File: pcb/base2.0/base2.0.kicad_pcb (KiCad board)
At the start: 4 copper layers, 24 x 24 mm, 33 parts, among them J1 Conn_01x01_Male, J2 Conn_01x01_Male, J3 Conn_ARM_JTAG_SWD_10, J4 Conn_01x02_Male, Q1 BSS123, U1 STM32G431CBU6, U2 tile, U3 AP2210-33, U4 LSM6DS3, U5 AP2210-5

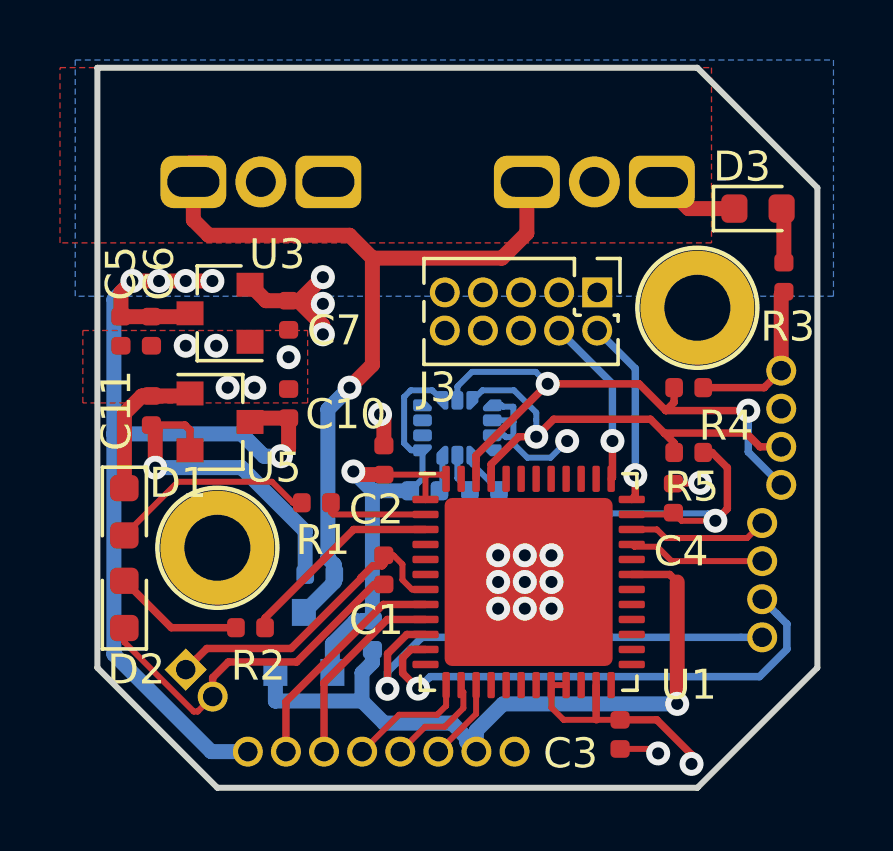
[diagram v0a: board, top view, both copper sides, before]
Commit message: added another pcbs
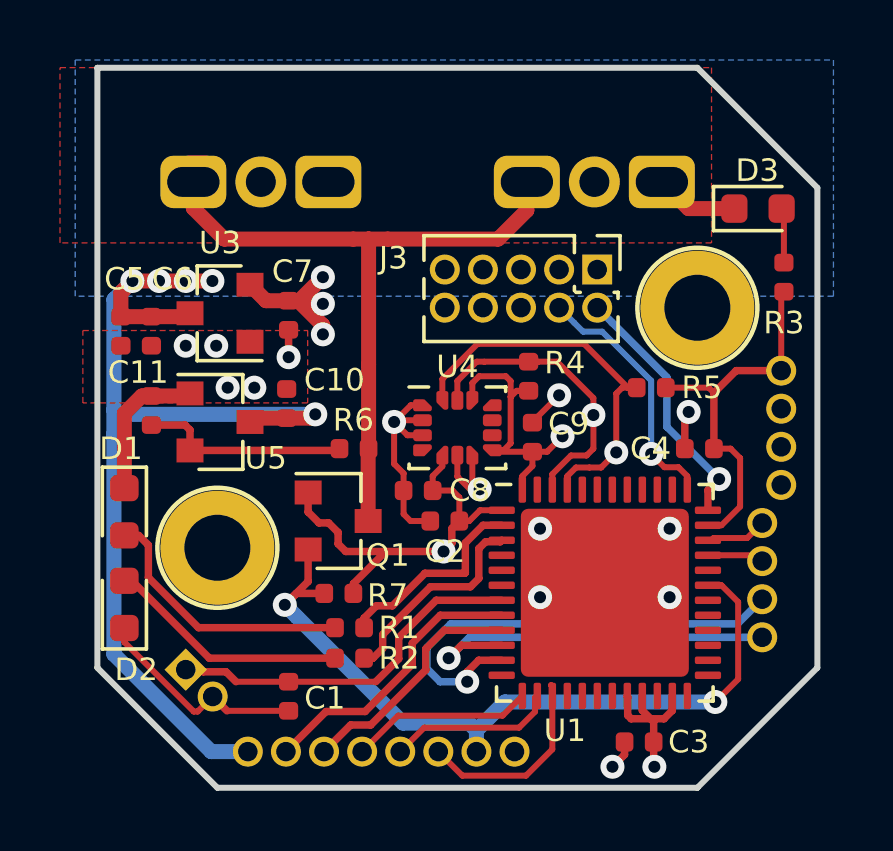
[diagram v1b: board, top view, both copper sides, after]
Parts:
- C8, C9, Q1, R6, R7, U4: moved to F.Cu
- moved R4 5.35 mm to (206.4, 97.3), turned to 90 degrees
- moved C1 5.28 mm to (198.4, 108.0)
- moved R6 4.34 mm to (200.6, 99.7)
- moved R1 4.31 mm to (200.4, 105.7)
- moved Q1 4.21 mm to (200.0, 102.1), turned to 0 degrees
- moved C9 4.00 mm to (206.5, 99.3), turned to 270 degrees
- moved R2 3.45 mm to (200.4, 106.7)
- moved C2 2.87 mm to (203.6, 102.1), turned to 180 degrees
- moved U1 2.57 mm to (208.9, 104.5)
- moved R5 2.49 mm to (210.5, 97.7)
- moved C8 2.21 mm to (202.7, 101.1)
- moved C4 1.86 mm to (212.1, 99.7), turned to 180 degrees
- moved R7 1.79 mm to (200.0, 104.5), turned to 180 degrees
- moved J3 0.76 mm to (208.7, 93.7)
- moved C3 0.68 mm to (210.1, 109.5), turned to 180 degrees
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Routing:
- net +3V3: track 54.1 -> 47.3 mm
- net USART1_5: track 28.4 -> 23.7 mm, vias 1 -> 0
- net I2C_SDA: track 15.3 -> 19.4 mm
- net GND: track 34.0 -> 30.1 mm, vias 18 -> 14
- net +5V: track 10.8 -> 7.04 mm, vias 1 -> 0
- net Net-(D2-Pad2): track 4.37 -> 8.09 mm
- net MOSI: track 2.74 -> 6.30 mm
- net USART2_TX: track 16.2 -> 12.7 mm
- net LED_2: track 3.50 -> 6.77 mm
- net JTCK-SWCLI: track 5.70 -> 8.48 mm
- net FDCAN_RX: track 4.58 -> 1.89 mm
- net FDCAN_TX: track 4.88 -> 2.26 mm
- net JTMS-SWDIO: track 6.21 -> 8.59 mm
- net MISO: track 3.51 -> 5.62 mm
- net SCK: track 4.12 -> 6.11 mm
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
